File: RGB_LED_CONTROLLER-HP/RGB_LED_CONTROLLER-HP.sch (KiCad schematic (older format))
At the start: 25 parts, among them J1 PWR IN, J2 PWM OUT, J3 AUX, Q1 IRF540N, Q2 IRF540N, Q3 IRF540N, SW1 SW_Push, U1 PIC12F629-IP, U1 PIC12F675-IP, U2 LM78L05_TO92

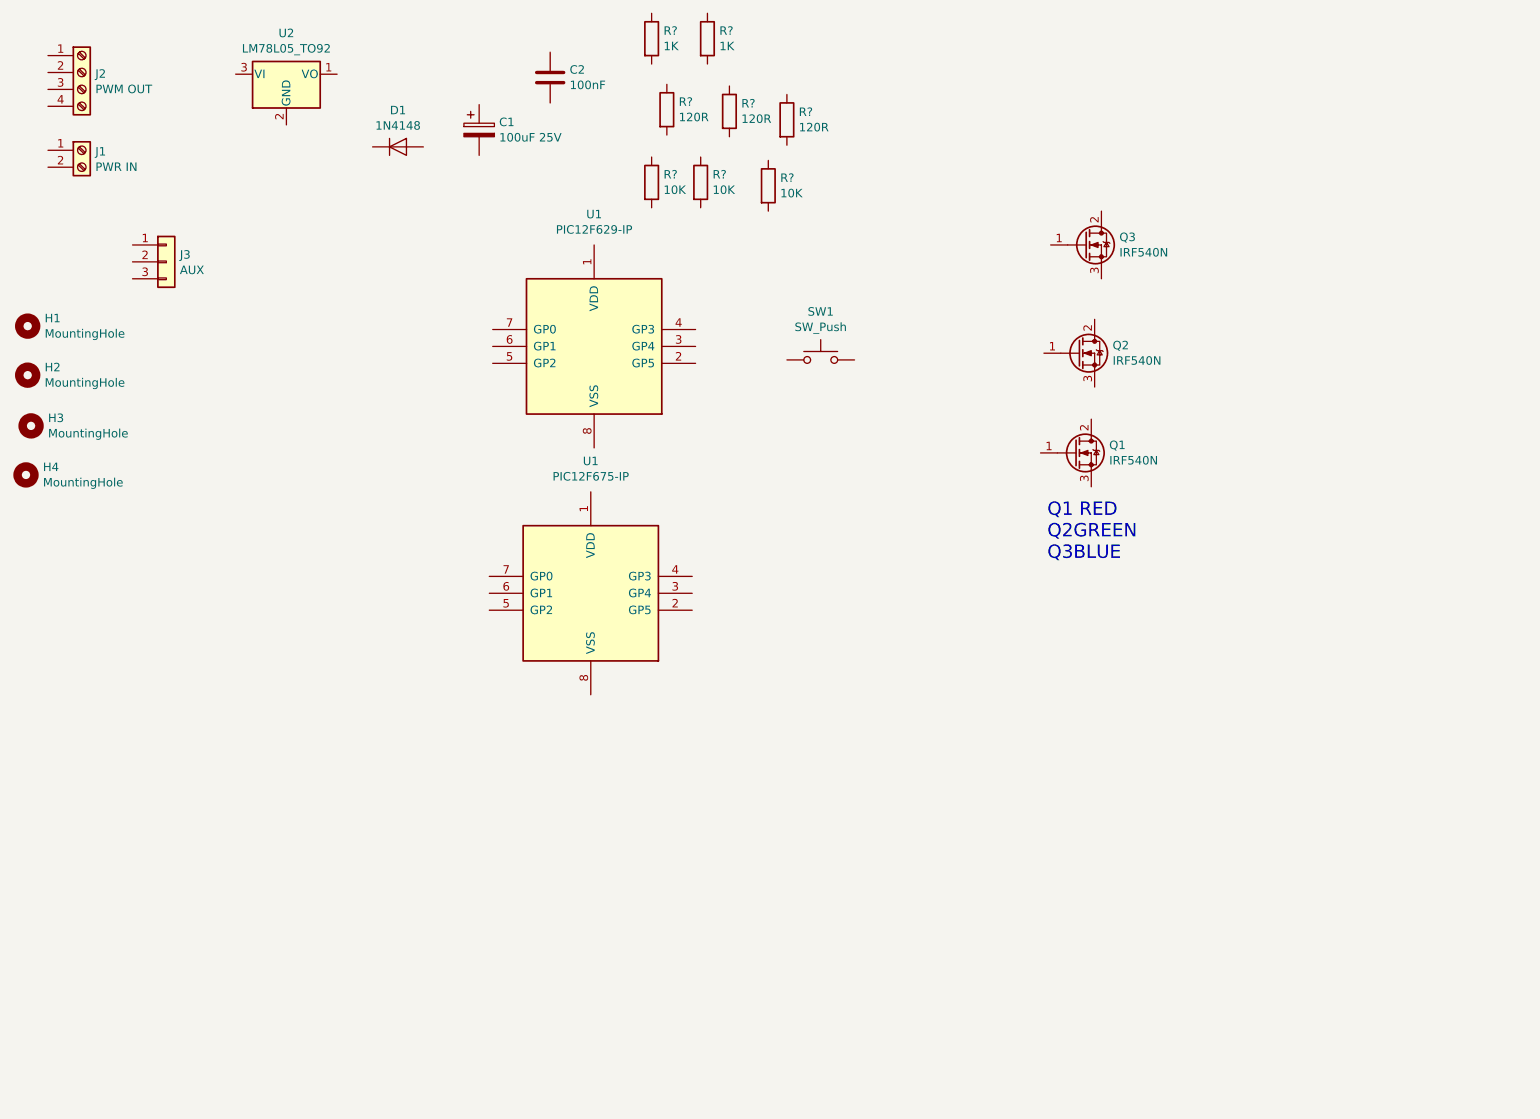
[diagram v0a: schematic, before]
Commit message: Second Commit
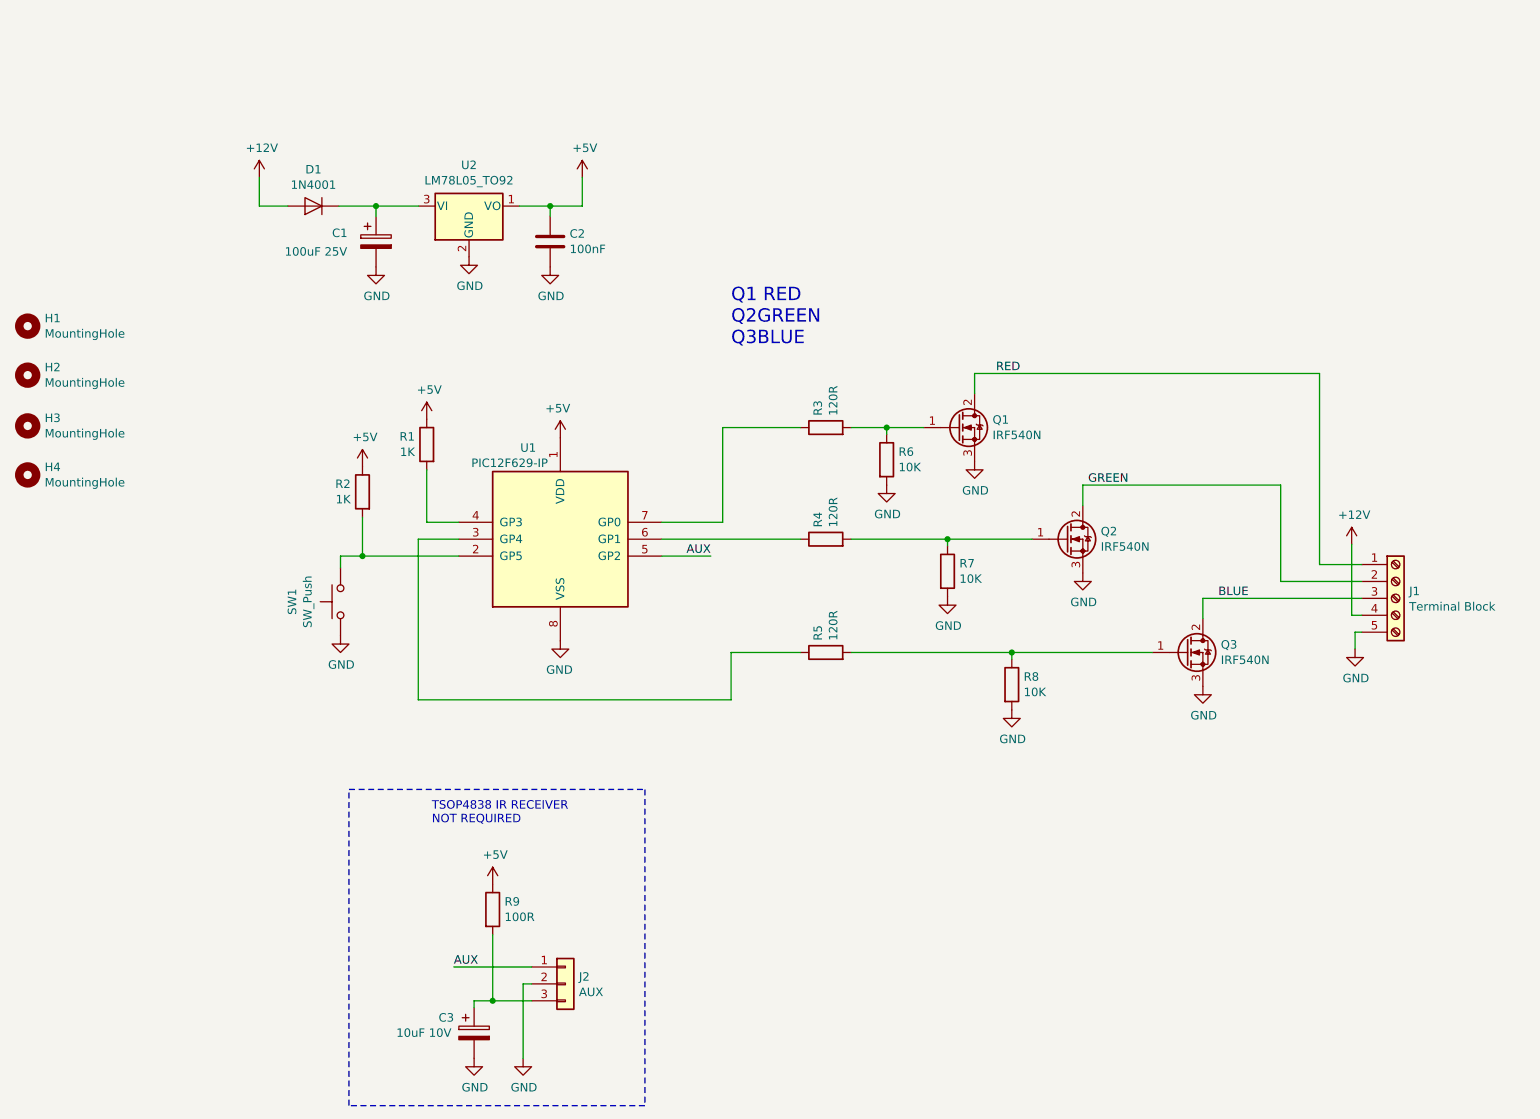
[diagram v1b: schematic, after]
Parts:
- removed D1: 1N4148, Diode_THT:D_DO-35_SOD27_P7.62mm_Horizontal, symbol Diode:1N4148
- removed J1: PWR IN, symbol Connector:Screw_Terminal_01x02
- removed J2: PWM OUT, symbol Connector:Screw_Terminal_01x04
- removed R? (x2): 10K, symbol Device:R
- removed U1: PIC12F675-IP, Package_DIP:DIP-8_W7.62mm, symbol MCU_Microchip_PIC12:PIC12F675-IP
- added C3: 10uF 10V, Capacitor_THT:CP_Radial_D5.0mm_P2.50mm, symbol Device:CP
- added D1: 1N4001, Diode_THT:D_DO-41_SOD81_P10.16mm_Horizontal, symbol Diode:1N4001
- added J1: Terminal Block, symbol Connector:Screw_Terminal_01x05
- added R7, R8: 10K, Resistor_THT:R_Axial_DIN0207_L6.3mm_D2.5mm_P10.16mm_Horizontal, symbol Device:R
- added R9: 100R, Resistor_THT:R_Axial_DIN0207_L6.3mm_D2.5mm_P10.16mm_Horizontal, symbol Device:R
- C1: footprint (none) -> Capacitor_THT:CP_Radial_D8.0mm_P3.50mm
- C2: footprint (none) -> Capacitor_THT:C_Disc_D3.0mm_W1.6mm_P2.50mm
- H1, H2, H3, H4: footprint (none) -> MountingHole:MountingHole_2.7mm_M2.5
- J2: renamed from J3; footprint (none) -> Connector_PinHeader_2.54mm:PinHeader_1x03_P2.54mm_Vertical
- R1, R2, R3, R4, R5, R6: renamed from R?; footprint (none) -> Resistor_THT:R_Axial_DIN0207_L6.3mm_D2.5mm_P10.16mm_Horizontal
- SW1: footprint (none) -> Button_Switch_THT:SW_Tactile_SPST_Angled_PTS645Vx83-2LFS
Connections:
- net +5V: now reaches U1.1 (VDD)
- net +5V: now also C2.1, R1.1, R2.1, U2.1 (VO), R9.1
- net at U1.2 (GP5): now also R2.2, SW1.2
- net at U1.3 (GP4): now also R5.1
- net at U1.4 (GP3): now also R1.2
- net AUX: now reaches U1.5 (GP2)
- net AUX: now also J2.1 (Pin_1)
- net at U1.6 (GP1): now also R4.1
- net at U1.7 (GP0): now also R3.1
- net GND: now reaches U1.8 (VSS)
- net GND: now also C1.2, C2.2, J2.2 (Pin_2), Q1.3 (S), Q2.3 (S), Q3.3 (S), R6.2, SW1.1, U2.2 (GND), C3.2, J1.5 (Pin_5), R7.2, R8.2
- net at C1.1: now also U2.3 (VI), D1.1 (K)
- net at J2.3 (Pin_3): now also C3.1, R9.2
- net at Q2.1 (G): now also R4.2, R7.1
- net GREEN: now reaches Q2.2 (D)
- net GREEN: now also J1.2 (Pin_2)
- net at Q1.1 (G): now also R3.2, R6.1
- net RED: now reaches Q1.2 (D)
- net RED: now also J1.1 (Pin_1)
- net at Q3.1 (G): now also R5.2, R8.1
- net BLUE: now reaches Q3.2 (D)
- net BLUE: now also J1.3 (Pin_3)
- new net +12V: D1.2 (A), J1.4 (Pin_4)
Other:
- note added: "TSOP4838 IR RECEIVER\nNOT REQUIRED"
- moved on the sheet: C1, C2, H3, J2, Q1, Q2, Q3, R1, R2, R3, R4, R5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
